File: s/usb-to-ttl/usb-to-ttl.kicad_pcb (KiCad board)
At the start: 2 copper layers, 25 x 16 mm, 9 parts, among them J1 USB_A, J2 Conn_01x05, U1 CH330N

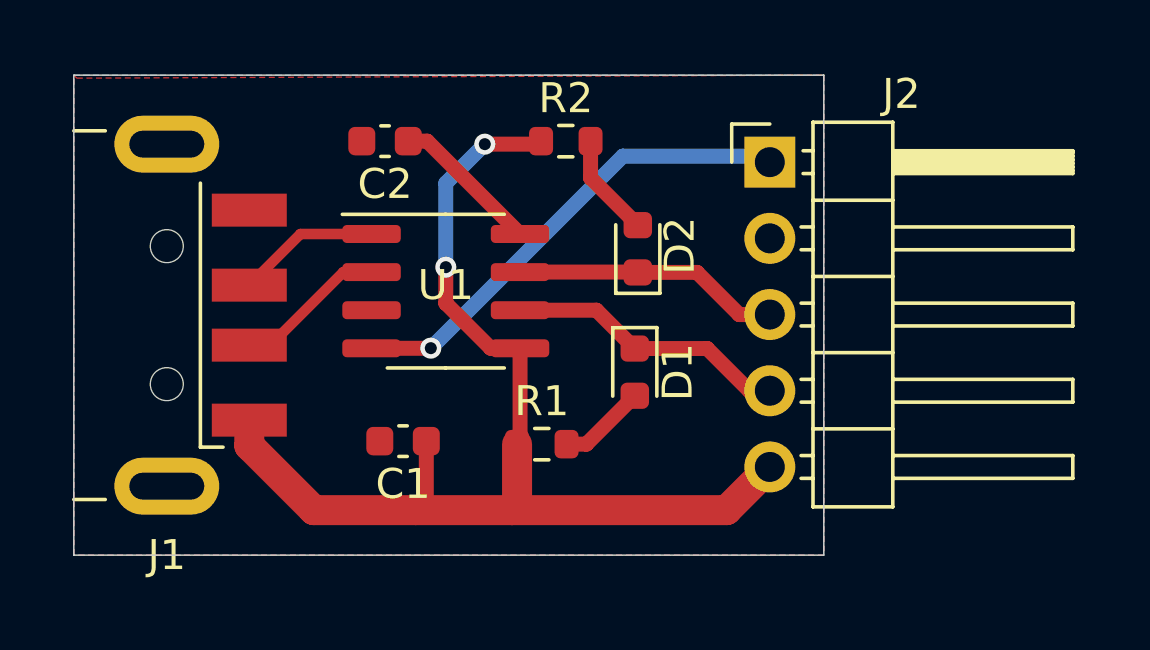
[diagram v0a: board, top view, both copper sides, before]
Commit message: 差分线 等长 等宽
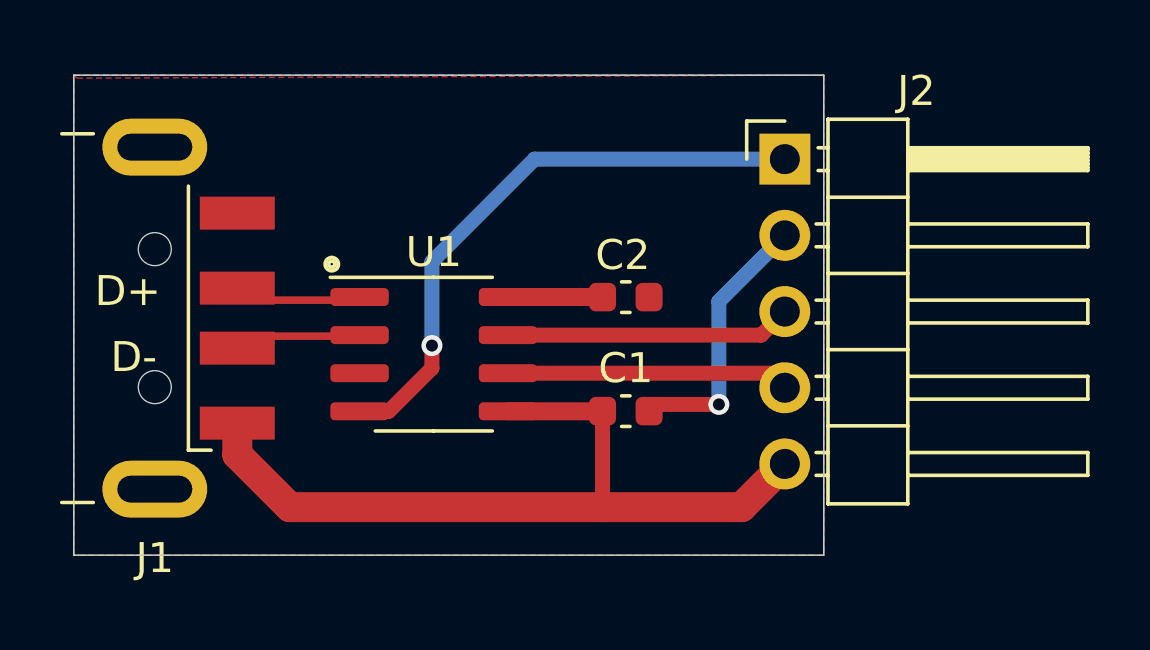
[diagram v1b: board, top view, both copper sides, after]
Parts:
- removed D1, D2: LED, LED_SMD:LED_0603_1608Metric
- removed R1, R2: 4.7k, Resistor_SMD:R_0603_1608Metric
- moved C2 9.56 mm to (118.4, 91.4), turned to 0 degrees
- moved C1 7.49 mm to (118.4, 95.2), turned to 0 degrees
- moved U1 2.14 mm to (112.0, 93.3)
- moved J2 0.51 mm to (123.7, 86.8)
- moved J1 0.41 mm to (95.8, 92.1)
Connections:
- net Net-(C2-Pad1) renamed /V3
- net Net-(D1-Pad1) renamed /TXD
- net Net-(D2-Pad1) renamed /RXD
- net Net-(J1-Pad2) renamed /D-
- net Net-(J1-Pad3) renamed /D+
- net Net-(J2-Pad1) renamed /RTS
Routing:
- net +5V: track 38.5 -> 27.0 mm, vias 2 -> 0
- net GND: track 0.00 -> 8.97 mm, vias 0 -> 1
- net /RTS: track 16.0 -> 19.9 mm
- net Net-(D2-Pad2): track 3.45 -> 0.00 mm
- net Net-(D1-Pad2): track 2.94 -> 0.00 mm
- net /V3: track 5.36 -> 3.15 mm
- net /D-: track 5.08 -> 4.26 mm
- net /RXD: track 8.91 -> 9.55 mm
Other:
- board text added: "D+"
- board text added: "D-"
